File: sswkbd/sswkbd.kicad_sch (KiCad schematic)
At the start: 238 parts, among them SW1 SW_PUSH, SW10 SW_PUSH, SW11 SW_PUSH, SW12 SW_PUSH, SW13 SW_PUSH, SW14 SW_PUSH, SW15 SW_PUSH, SW16 SW_PUSH, SW17 SW_PUSH, SW18 SW_PUSH, SW19 SW_PUSH, SW2 SW_PUSH, SW20 SW_PUSH, SW21 SW_PUSH, SW22 SW_PUSH, SW23 SW_PUSH, SW24 SW_PUSH, SW25 SW_PUSH, SW26 SW_PUSH, SW27 SW_PUSH, SW28 SW_PUSH, SW29 SW_PUSH, SW3 SW_PUSH, SW30 SW_PUSH, SW31 SW_PUSH, SW32 SW_PUSH, SW33 SW_PUSH, SW34 SW_PUSH, SW35 SW_PUSH, SW36 SW_PUSH, SW37 SW_PUSH, SW38 SW_PUSH, SW39 SW_PUSH, SW4 SW_PUSH, SW40 SW_PUSH, SW41 SW_PUSH, SW42 SW_PUSH, SW43 SW_PUSH, SW44 SW_PUSH, SW45 SW_PUSH, SW46 SW_PUSH, SW47 SW_PUSH, SW48 SW_PUSH, SW49 SW_PUSH, SW5 SW_PUSH, SW50 SW_PUSH, SW51 SW_PUSH, SW52 SW_PUSH, SW53 SW_PUSH, SW54 SW_PUSH, SW55 SW_PUSH, SW56 SW_PUSH, SW57 SW_PUSH, SW58 SW_PUSH, SW59 SW_PUSH, SW6 SW_PUSH, SW60 SW_PUSH, SW61 SW_PUSH, SW62 SW_PUSH, SW63 SW_PUSH, SW64 SW_PUSH, SW65 SW_PUSH, SW66 SW_PUSH, SW67 SW_PUSH, SW68 SW_PUSH, SW69 SW_PUSH, SW7 SW_PUSH, SW70 SW_PUSH, SW71 SW_PUSH, SW72 SW_PUSH, SW73 SW_PUSH, SW74 SW_PUSH, SW75 SW_PUSH, SW76 SW_PUSH, SW77 SW_PUSH, SW78 SW_PUSH, SW79 SW_PUSH, SW8 SW_PUSH, SW9 SW_PUSH, U1 ProMicro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

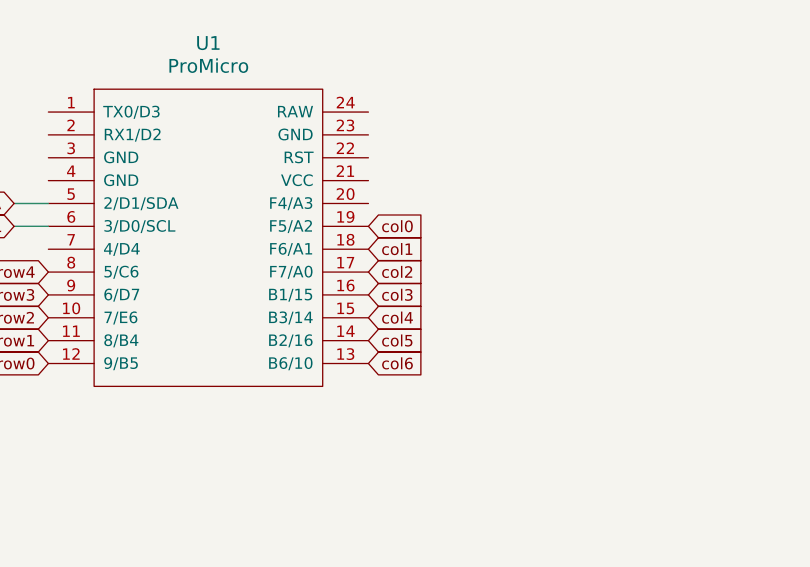
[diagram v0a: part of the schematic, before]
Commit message: update
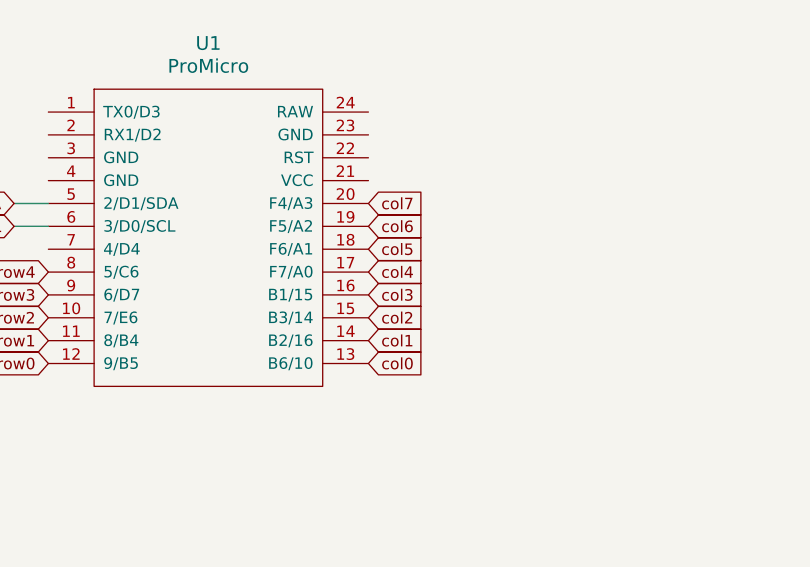
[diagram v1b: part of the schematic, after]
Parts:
- LED1, LED10, LED11, LED12, LED13, LED14, LED15, LED16, LED17, LED18, LED19, LED2, LED20, LED21, LED22, LED23, LED24, LED25, LED26, LED27, LED28, LED29, LED3, LED30, LED31, LED32, LED33, LED34, LED35, LED36, LED37, LED38, LED39, LED4, LED40, LED41, LED42, LED43, LED44, LED45, LED46, LED47, LED48, LED49, LED5, LED50, LED51, LED52, LED53, LED54, LED55, LED56, LED57, LED58, LED59, LED6, LED60, LED61, LED62, LED63, LED64, LED65, LED66, LED67, LED68, LED69, LED7, LED70, LED71, LED72, LED73, LED74, LED75, LED76, LED77, LED78, LED8, LED9: footprint (none) -> kbd:SK6812MINI-E
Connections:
- net col0: now also U1.13 (B6/10); no longer U1.19 (F5/A2)
- net col1: now also U1.14 (B2/16); no longer U1.18 (F6/A1)
- net col2: now also U1.15 (B3/14); no longer U1.17 (F7/A0)
- net col4: now also U1.17 (F7/A0); no longer U1.15 (B3/14)
- net col5: now also U1.18 (F6/A1); no longer U1.14 (B2/16)
- net col6: now also U1.19 (F5/A2); no longer U1.13 (B6/10)
- net col7: now also U1.20 (F4/A3)

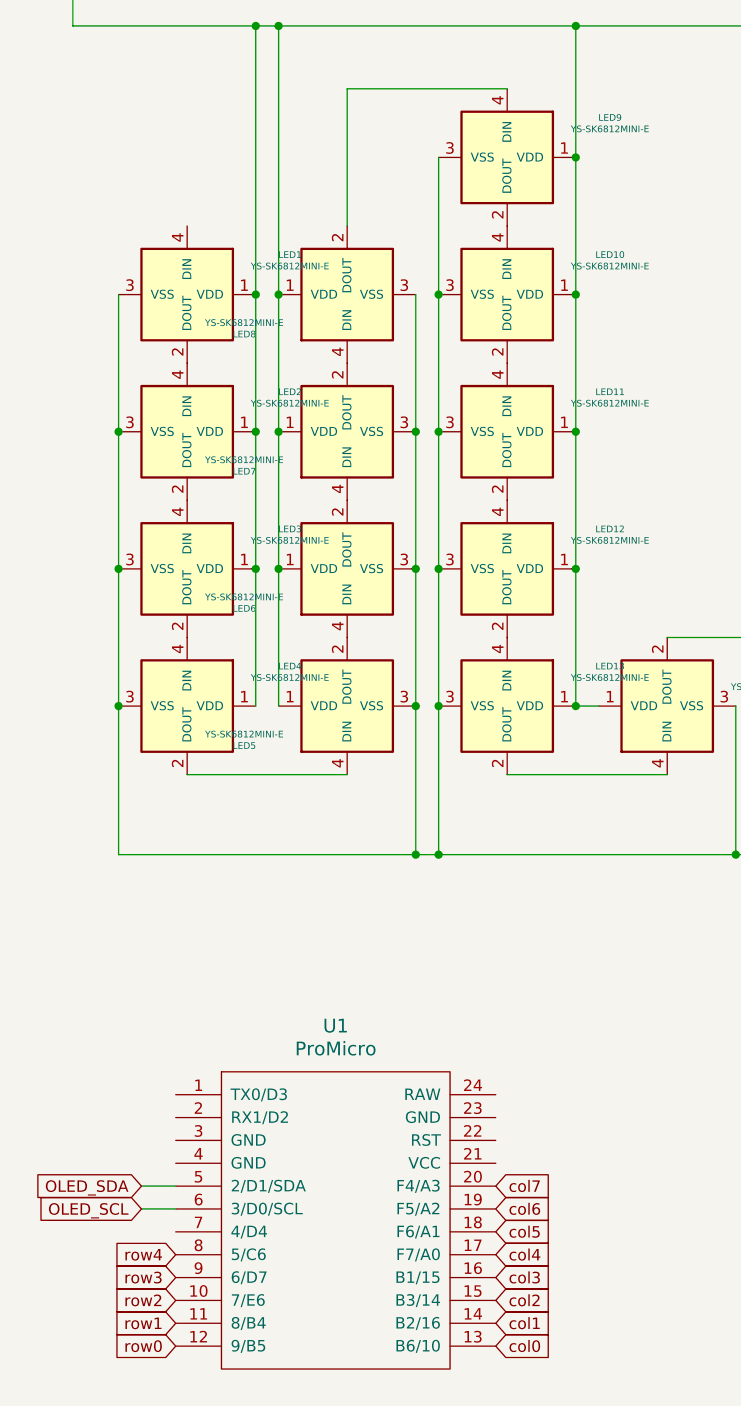
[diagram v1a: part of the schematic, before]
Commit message: PCB WIP
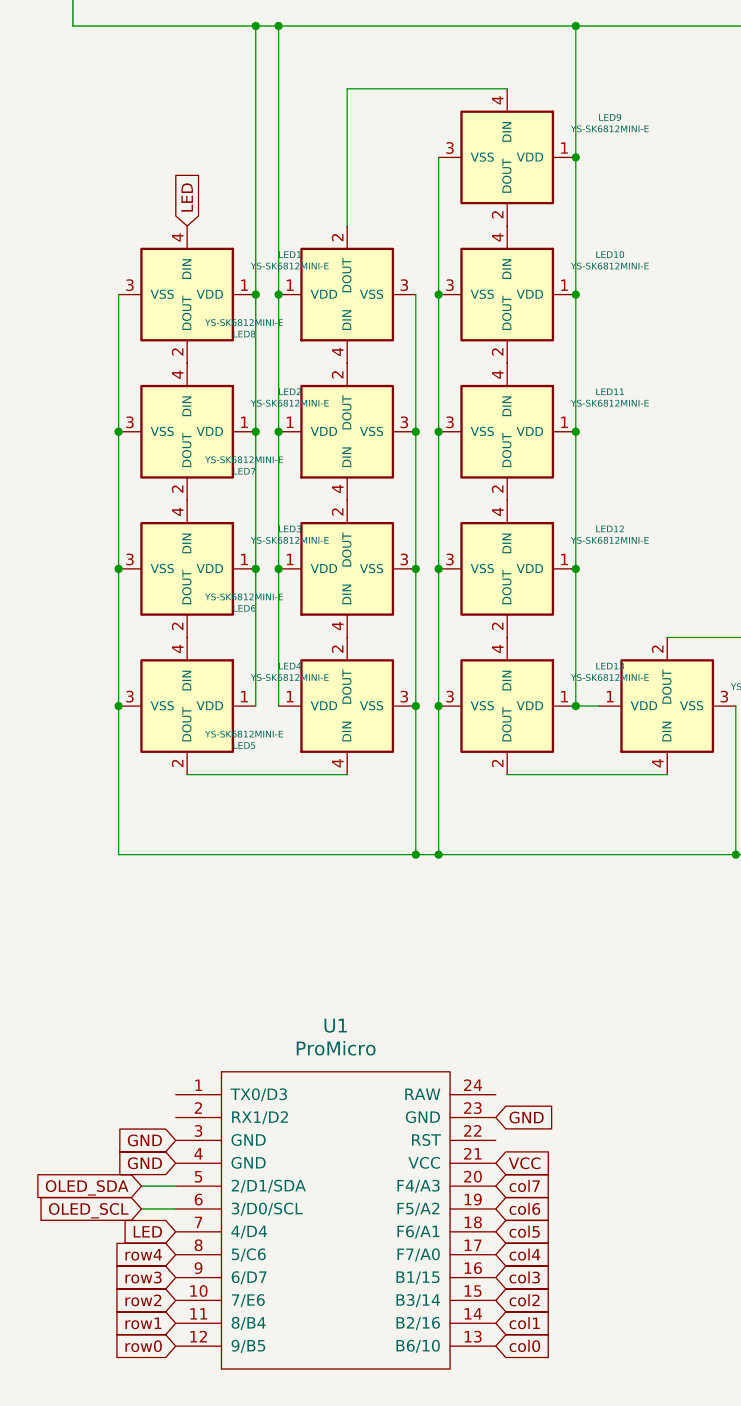
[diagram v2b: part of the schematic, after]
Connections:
- net GND: now also U1.23 (GND), U1.3 (GND), U1.4 (GND)
- net VCC: now also U1.21 (VCC)
- net LED: now reaches LED1.4 (DIN)
- net LED: now also U1.7 (4/D4)
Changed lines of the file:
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@@
+		)
+	)
+	(global_label "LED"
+		(shape input)
+		(at 31.75 262.89 180)
+		(fields_autoplaced yes)
+		(effects
+			(font
+				(size 1.27 1.27)
+			)
+			(justify right)
+		)
+		(property "Intersheetrefs" "${INTERSHEET_REFS}"
+			(at 25.3177 262.89 0)
+			(effects
+				(font
+					(size 1.27 1.27)
+				)
+				(justify right)
+				(hide yes)
+			)
+		)
+	)
+	(global_label "GND"
+		(shape input)
+		(at 31.75 255.27 180)
+		(fields_autoplaced yes)
+		(effects
+			(font
+				(size 1.27 1.27)
+			)
+			(justify right)
+		)
+		(property "Intersheetrefs" "${INTERSHEET_REFS}"
+			(at 24.8943 255.27 0)
+			(effects
+				(font
+					(size 1.27 1.27)
+				)
+				(justify right)
+				(hide yes)
+			)
 		)
 	)
@@
 		)
 	)
+	(global_label "GND"
+		(shape input)
+		(at 67.31 250.19 0)
+		(fields_autoplaced yes)
+		(effects
+			(font
+				(size 1.27 1.27)
+			)
+			(justify left)
+		)
+		(property "Intersheetrefs" "${INTERSHEET_REFS}"
+			(at 74.1657 250.19 0)
+			(effects
+				(font
+					(size 1.27 1.27)
+				)
+				(justify left)
+				(hide yes)
+			)
+		)
+	)
 	(global_label "row0"
 		(shape input)
@@
 		)
 	)
+	(global_label "GND"
+		(shape input)
+		(at 31.75 252.73 180)
+		(fields_autoplaced yes)
+		(effects
+			(font
+				(size 1.27 1.27)
+			)
+			(justify right)
+		)
+		(property "Intersheetrefs" "${INTERSHEET_REFS}"
+			(at 24.8943 252.73 0)
+			(effects
+				(font
+					(size 1.27 1.27)
+				)
+				(justify right)
+				(hide yes)
+			)
+		)
+	)
 	(global_label "col7"
 		(shape input)
@@
 		)
 	)
+	(global_label "LED"
+		(shape input)
+		(at 33.02 151.13 90)
+		(fields_autoplaced yes)
+		(effects
+			(font
+				(size 1.27 1.27)
+			)
+			(justify left)
+		)
+		(property "Intersheetrefs" "${INTERSHEET_REFS}"
+			(at 33.02 144.6977 90)
+			(effects
+				(font
+					(size 1.27 1.27)
+				)
+				(justify left)
+				(hide yes)
+			)
+		)
+	)
 	(global_label "col_r_5"
 		(shape input)
@@
 			(effects
 				(font
+					(size 1.27 1.27)
+				)
+				(justify left)
+				(hide yes)
+			)
+		)
+	)
+	(global_label "VCC"
+		(shape input)
+		(at 67.31 255.27 0)
+		(fields_autoplaced yes)
+		(effects
+			(font
+				(size 1.27 1.27)
+			)
+			(justify left)
+		)
+		(property "Intersheetrefs" "${INTERSHEET_REFS}"
+			(at 73.9238 255.27 0)
+			(effects
+				(font
